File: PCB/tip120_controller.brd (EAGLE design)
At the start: 52.4 x 37.5 mm, 14 parts, among them J1 AUDIO_JACK_3.5MM_PTH, Q1 TIP120, U1 ARDUINO_MINI

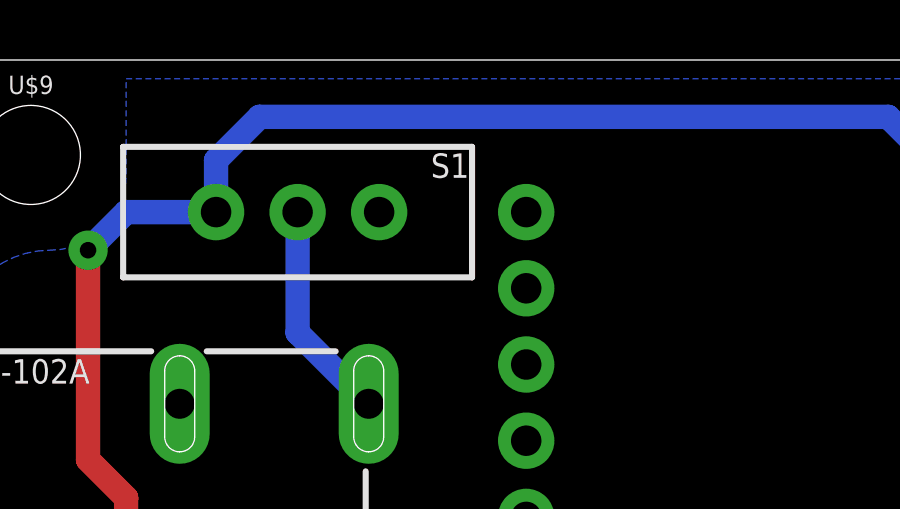
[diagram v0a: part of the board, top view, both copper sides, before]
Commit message: sanity check
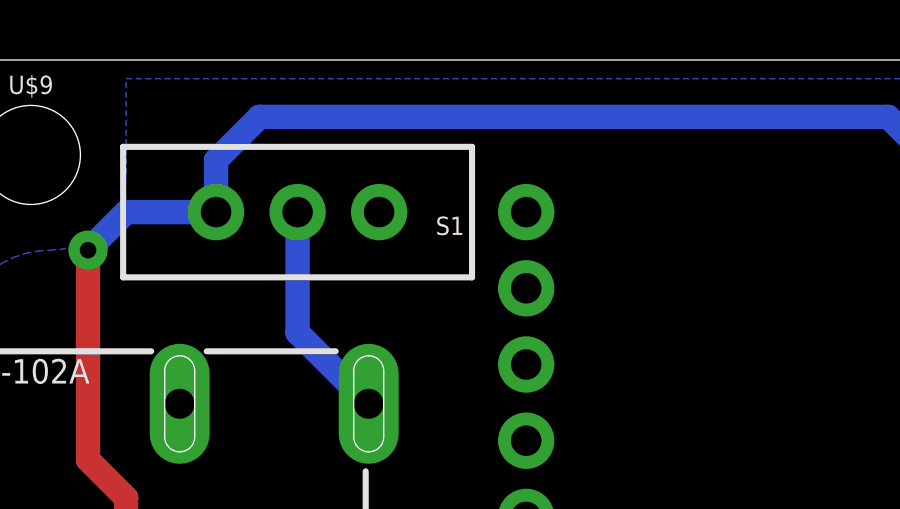
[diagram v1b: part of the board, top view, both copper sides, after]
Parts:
- LED1: value (none) -> RED
- S1: value 6-12V -> EG1218
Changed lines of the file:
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@@
 <attribute name="VALUE" x="0.635" y="71.755" size="0.8128" layer="27" font="vector" ratio="15"/>
-</element>
-<element name="S1" library="SparkFun-Switches" package="SWITCH_SPDT_PTH_11.6X4.0MM_KIT" value="6-12V" x="11.43" y="78.74" smashed="yes" rot="R270">
-<attribute name="NAME" x="16.51" y="79.883" size="0.8128" layer="25" font="vector" ratio="15" align="bottom-center"/>
-<attribute name="PROD_ID" value="SWCH-08261" x="11.43" y="78.74" size="1.778" layer="27" rot="R270" display="off"/>
-<attribute name="SF_SKU" value="COM-00102" x="11.43" y="78.74" size="1.778" layer="27" rot="R270" display="off"/>
 </element>
 <element name="R2" library="resistor" library_urn="urn:adsk.eagle:library:348" package="0204V" package3d_urn="urn:adsk.eagle:package:25948/1" value="220" x="38.1" y="78.74" smashed="yes" rot="R180">
 <attribute name="NAME" x="38.9636" y="80.7466" size="0.8128" layer="25" font="vector" ratio="15" rot="R180"/>
 </element>
-<element name="LED1" library="led" library_urn="urn:adsk.eagle:library:259" package="LED5MM" package3d_urn="urn:adsk.eagle:package:15799/2" value="" x="39.37" y="74.295" smashed="yes" rot="R270">
+<element name="LED1" library="led" library_urn="urn:adsk.eagle:library:259" package="LED5MM" package3d_urn="urn:adsk.eagle:package:15799/2" value="RED" x="39.37" y="74.295" smashed="yes" rot="R270">
 <attribute name="NAME" x="38.735" y="70.3834" size="0.8128" layer="25" font="vector" ratio="15"/>
 </element>
@@
 <element name="Q1" library="transistor-power" library_urn="urn:adsk.eagle:library:400" package="TO220AV" package3d_urn="urn:adsk.eagle:package:29487/2" value="TIP120" x="12.7" y="59.055" smashed="yes" rot="R90">
 <attribute name="NAME" x="15.875" y="63.8302" size="0.8128" layer="25" font="vector" ratio="15" rot="R180"/>
+</element>
+<element name="S1" library="SparkFun-Switches" package="SWITCH_SPDT_PTH_11.6X4.0MM_KIT" value="EG1218" x="11.43" y="78.74" smashed="yes" rot="R270">
+<attribute name="NAME" x="16.51" y="77.978" size="0.6096" layer="25" font="vector" ratio="20" align="bottom-center"/>
+<attribute name="PROD_ID" value="SWCH-08261" x="11.43" y="78.74" size="1.778" layer="27" rot="R270" display="off"/>
+<attribute name="SF_SKU" value="COM-00102" x="11.43" y="78.74" size="1.778" layer="27" rot="R270" display="off"/>
+<attribute name="VALUE" x="15.24" y="77.597" size="0.6096" layer="27" font="vector" ratio="20" align="top-center"/>
 </element>
 </elements>
@@
 <signal name="N$7">
 <contactref element="PJ-102A" pad="1"/>
+<wire x1="13.8" y1="72.35" x2="11.43" y2="74.72" width="0.8128" layer="16"/>
 <contactref element="S1" pad="2"/>
-<wire x1="13.8" y1="72.35" x2="11.43" y2="74.72" width="0.8128" layer="16"/>
 <wire x1="11.43" y1="74.72" x2="11.43" y2="78.74" width="0.8128" layer="16"/>
 </signal>
 <signal name="N$8">
-<contactref element="S1" pad="3"/>
 <contactref element="R2" pad="2"/>
 <contactref element="U1" pad="24"/>
@@
 <wire x1="8.175" y1="54.055" x2="8.255" y2="53.975" width="0.8128" layer="16"/>
 <wire x1="8.255" y1="53.975" x2="12.065" y2="53.975" width="0.8128" layer="16"/>
-<wire x1="8.7122" y1="78.74" x2="8.7122" y2="80.4672" width="0.8128" layer="16"/>
 <wire x1="8.7122" y1="80.4672" x2="10.16" y2="81.915" width="0.8128" layer="16"/>
 <wire x1="10.16" y1="81.915" x2="31.115" y2="81.915" width="0.8128" layer="16"/>
@@
 <wire x1="4.445" y1="70.485" x2="4.445" y2="77.47" width="0.8128" layer="1"/>
 <wire x1="4.445" y1="77.47" x2="5.715" y2="78.74" width="0.8128" layer="16"/>
+<contactref element="S1" pad="3"/>
 <wire x1="5.715" y1="78.74" x2="8.7122" y2="78.74" width="0.8128" layer="16"/>
+<wire x1="8.7122" y1="78.74" x2="8.7122" y2="80.4672" width="0.8128" layer="16"/>
 </signal>
 <signal name="N$1">
